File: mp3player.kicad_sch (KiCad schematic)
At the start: 7 parts, among them J1 AudioJack3, U1 ES8388, U2 ESP32-S3-WROOM-1

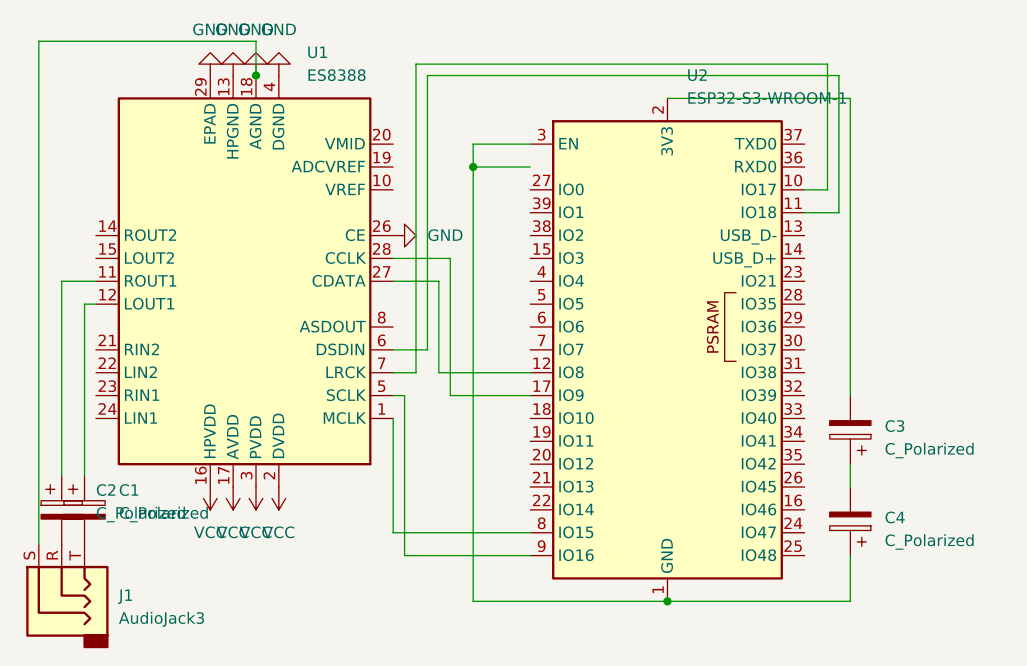
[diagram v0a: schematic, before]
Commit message: Autosave
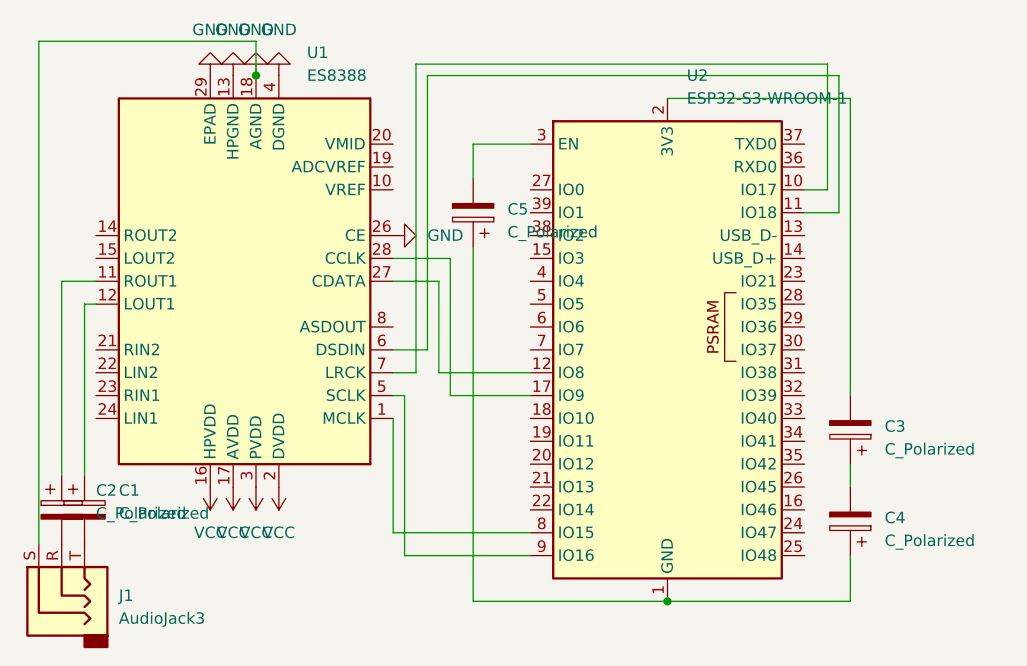
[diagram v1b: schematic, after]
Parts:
- added C5: C_Polarized, symbol Device:C_Polarized
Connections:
- net at C4.1, U2.1 (GND), U2.40 (GND)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: now also C5.1; no longer U2.3 (EN)
- new net: C5.2, U2.3 (EN)
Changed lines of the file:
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@@
-	)
-	(junction
-		(at 63.5 26.67)
-		(diameter 0)
-		(color 0 0 0 0)
 	)
 	(junction
@@
 	(wire
 		(pts
-			(xy 69.85 26.67) (xy 63.5 26.67)
-		)
-		(stroke
-			(width 0)
-			(type default)
-		)
-	)
-	(wire
-		(pts
 			(xy 54.61 36.83) (xy 60.96 36.83)
 		)
@@
 	(wire
 		(pts
-			(xy 63.5 24.13) (xy 63.5 26.67)
+			(xy 63.5 35.56) (xy 63.5 74.93)
 		)
 		(stroke
@@
 	(wire
 		(pts
-			(xy 63.5 26.67) (xy 63.5 74.93)
+			(xy 63.5 24.13) (xy 63.5 27.94)
 		)
 		(stroke
@@
 					(unit 1)
 				)
+			)
+		)
+	)
+	(symbol
+		(lib_id "Device:C_Polarized")
+		(at 63.5 31.75 180)
+		(unit 1)
+		(body_style 1)
+		(exclude_from_sim no)
+		(in_bom yes)
+		(on_board yes)
+		(in_pos_files yes)
+		(dnp no)
+		(fields_autoplaced yes)
+		(property "Reference" "C5"
+			(at 67.31 31.3689 0)
+			(show_name no)
+			(do_not_autoplace no)
+			(effects
+				(font
+					(size 1.27 1.27)
+				)
+				(justify right)
+			)
+		)
+		(property "Value" "C_Polarized"
+			(at 67.31 33.9089 0)
+			(show_name no)
+			(do_not_autoplace no)
+			(effects
+				(font
+					(size 1.27 1.27)
+				)
+				(justify right)
+			)
+		)
+		(property "Footprint" ""
+			(at 62.5348 27.94 0)
+			(hide yes)
+			(show_name no)
+			(do_not_autoplace no)
+			(effects
+				(font
+					(size 1.27 1.27)
+				)
+			)
+		)
+		(property "Datasheet" ""
+			(at 63.5 31.75 0)
+			(hide yes)
+			(show_name no)
+			(do_not_autoplace no)
+			(effects
+				(font
+					(size 1.27 1.27)
+				)
+			)
+		)
+		(property "Description" "Polarized capacitor"
+			(at 63.5 31.75 0)
+			(hide yes)
+			(show_name no)
+			(do_not_autoplace no)
+			(effects
+				(font
+					(size 1.27 1.27)
+				)
+			)
+		)
+		(pin "1"
+		)
+		(pin "2"
+		)
+		(instances
+			(project "mp3player"
+				(path "/7851373b-cb7e-4e42-801a-d8b5ac5735f4"
+					(reference "C5")
+					(unit 1)
+				)

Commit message: Autosave
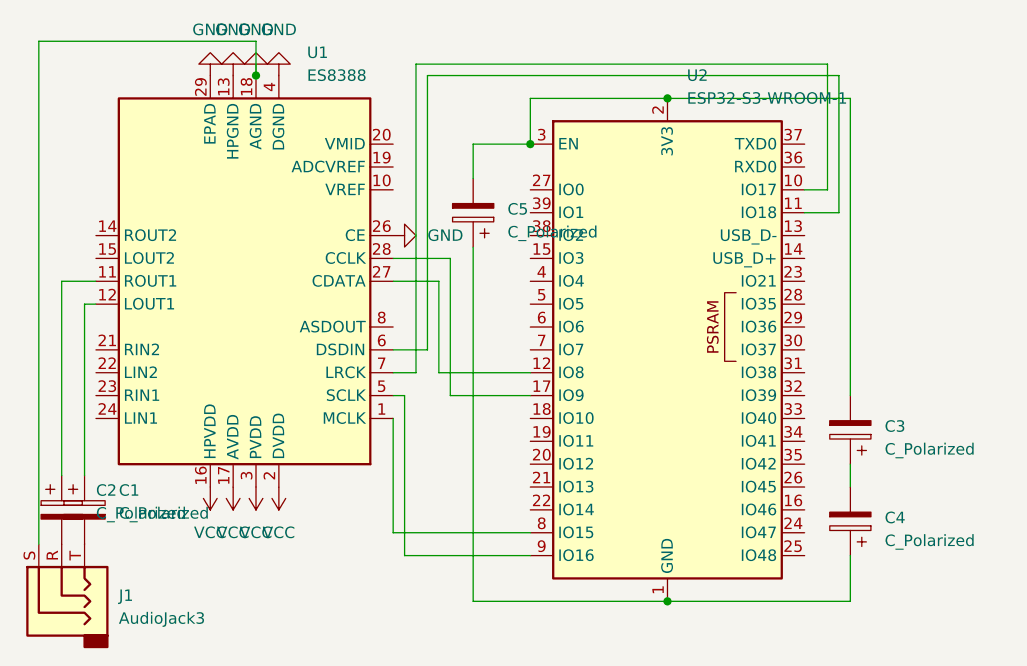
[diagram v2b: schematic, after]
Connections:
- net at C5.2, U2.3 (EN): now also C3.2, U2.2 (3V3)
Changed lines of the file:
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@@
 	(paper "A4")
 	(junction
+		(at 85.09 19.05)
+		(diameter 0)
+		(color 0 0 0 0)
+	)
+	(junction
 		(at 39.37 16.51)
 		(diameter 0)
@@
 	)
 	(junction
+		(at 69.85 24.13)
+		(diameter 0)
+		(color 0 0 0 0)
+	)
+	(junction
 		(at 85.09 74.93)
 		(diameter 0)
@@
 	(wire
 		(pts
+			(xy 69.85 19.05) (xy 85.09 19.05)
+		)
+		(stroke
+			(width 0)
+			(type default)
+		)
+	)
+	(wire
+		(pts
 			(xy 100.33 31.75) (xy 104.14 31.75)
 		)
@@
 		)
 		(stroke
+			(width 0)
+			(type default)
+		)
+	)
+	(wire
+		(pts
+			(xy 69.85 24.13) (xy 69.85 19.05)
+		)
+		(stroke

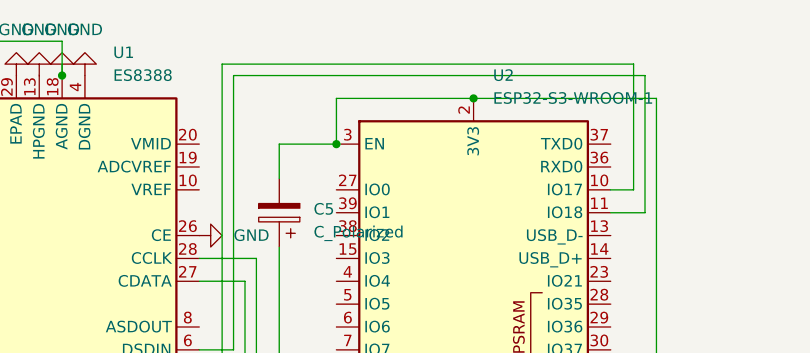
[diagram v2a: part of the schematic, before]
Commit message: Autosave
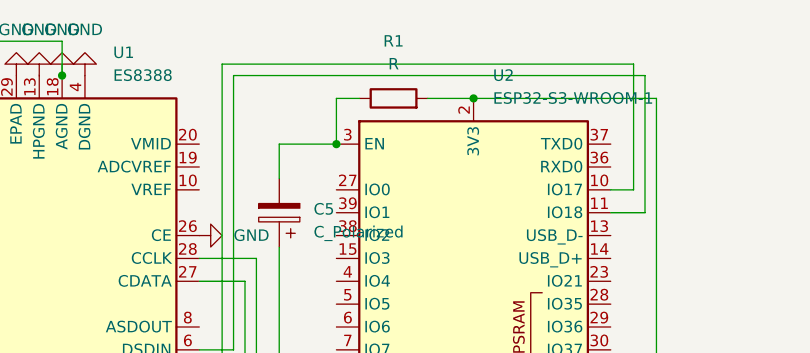
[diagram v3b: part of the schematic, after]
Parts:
- added R1: R, symbol Device:R
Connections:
- net at C5.2, U2.3 (EN): now also R1.1; no longer C3.2, U2.2 (3V3)
- new net: C3.2, R1.2, U2.2 (3V3)
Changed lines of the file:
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@@
 	(wire
 		(pts
-			(xy 69.85 19.05) (xy 85.09 19.05)
+			(xy 69.85 19.05) (xy 72.39 19.05)
 		)
 		(stroke
@@
 		(pts
 			(xy 63.5 24.13) (xy 63.5 27.94)
+		)
+		(stroke
+			(width 0)
+			(type default)
+		)
+	)
+	(wire
+		(pts
+			(xy 80.01 19.05) (xy 85.09 19.05)
 		)
 		(stroke
@@
 					(unit 1)
 				)
+			)
+		)
+	)
+	(symbol
+		(lib_id "Device:R")
+		(at 76.2 19.05 90)
+		(unit 1)
+		(body_style 1)
+		(exclude_from_sim no)
+		(in_bom yes)
+		(on_board yes)
+		(in_pos_files yes)
+		(dnp no)
+		(fields_autoplaced yes)
+		(property "Reference" "R1"
+			(at 76.2 12.7 90)
+			(show_name no)
+			(do_not_autoplace no)
+			(effects
+				(font
+					(size 1.27 1.27)
+				)
+			)
+		)
+		(property "Value" "R"
+			(at 76.2 15.24 90)
+			(show_name no)
+			(do_not_autoplace no)
+			(effects
+				(font
+					(size 1.27 1.27)
+				)
+			)
+		)
+		(property "Footprint" ""
+			(at 76.2 20.828 90)
+			(hide yes)
+			(show_name no)
+			(do_not_autoplace no)
+			(effects
+				(font
+					(size 1.27 1.27)
+				)
+			)
+		)
+		(property "Datasheet" ""
+			(at 76.2 19.05 0)
+			(hide yes)
+			(show_name no)
+			(do_not_autoplace no)
+			(effects
+				(font
+					(size 1.27 1.27)
+				)
+			)
+		)
+		(property "Description" "Resistor"
+			(at 76.2 19.05 0)
+			(hide yes)
+			(show_name no)
+			(do_not_autoplace no)
+			(effects
+				(font
+					(size 1.27 1.27)
+				)
+			)
+		)
+		(pin "1"
+		)
+		(pin "2"
+		)
+		(instances
+			(project "mp3player"
+				(path "/7851373b-cb7e-4e42-801a-d8b5ac5735f4"
+					(reference "R1")
+					(unit 1)
+				)

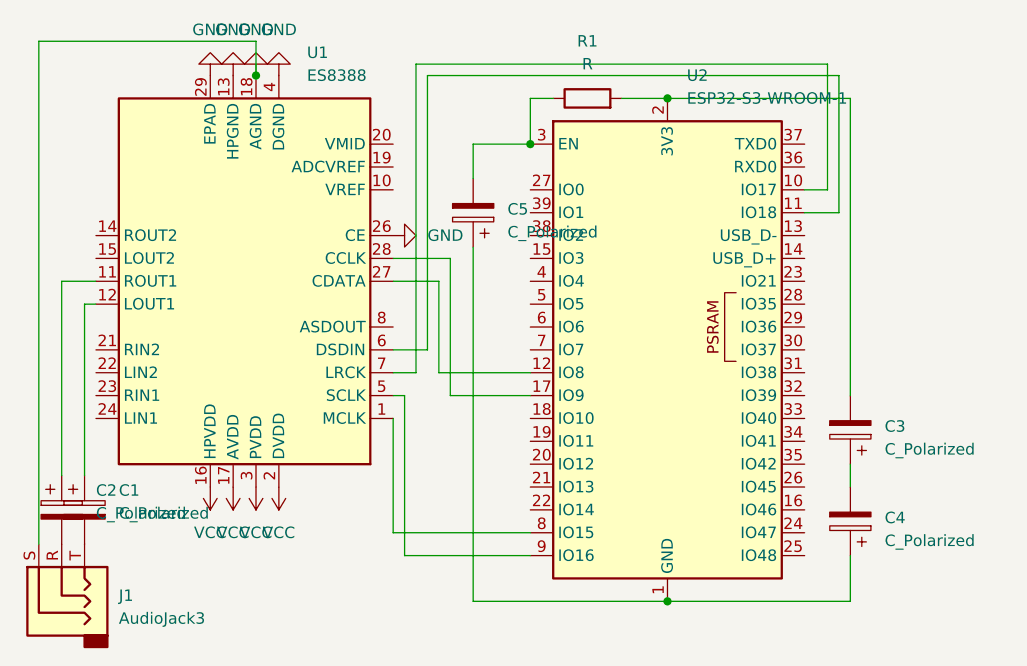
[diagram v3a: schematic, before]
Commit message: Autosave
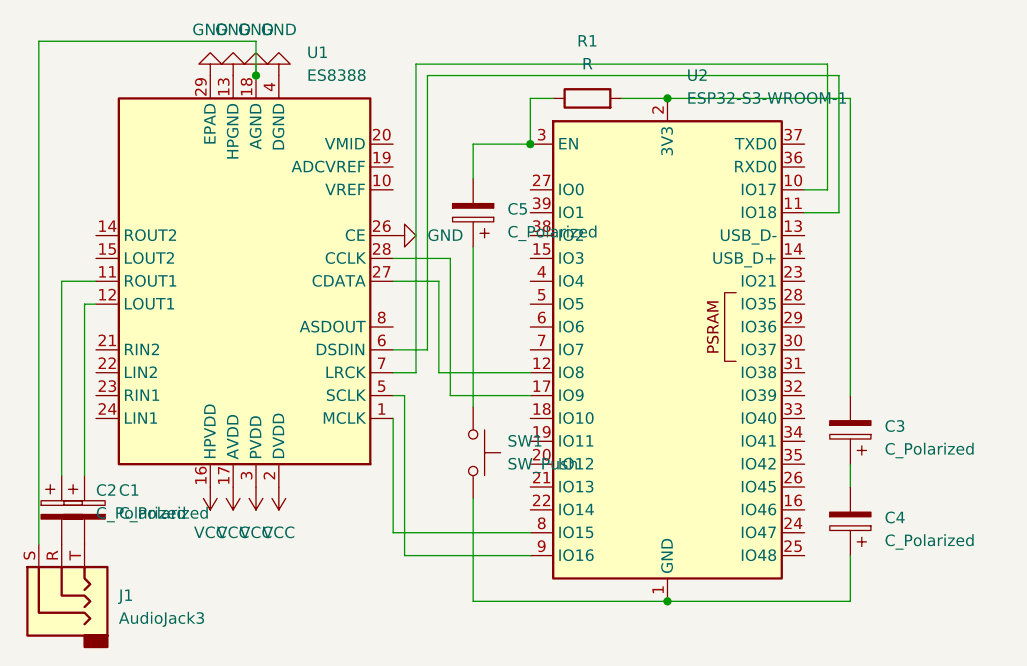
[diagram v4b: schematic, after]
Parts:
- added SW1: SW_Push, symbol Switch:SW_Push
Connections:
- net at C4.1, U2.1 (GND), U2.40 (GND)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: now also SW1.2; no longer C5.1
- new net: C5.1, SW1.1
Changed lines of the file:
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@@
+	(wire
+		(pts
+			(xy 63.5 63.5) (xy 63.5 74.93)
+		)
+		(stroke
+			(width 0)
+			(type default)
+		)
+	)
 	(wire
 		(pts
@@
 	(wire
 		(pts
-			(xy 63.5 35.56) (xy 63.5 74.93)
+			(xy 63.5 35.56) (xy 63.5 53.34)
 		)
 		(stroke
@@
 					(unit 1)
 				)
+			)
+		)
+	)
+	(symbol
+		(lib_id "Switch:SW_Push")
+		(at 63.5 58.42 270)
+		(unit 1)
+		(body_style 1)
+		(exclude_from_sim no)
+		(in_bom yes)
+		(on_board yes)
+		(in_pos_files yes)
+		(dnp no)
+		(fields_autoplaced yes)
+		(property "Reference" "SW1"
+			(at 67.31 57.1499 90)
+			(show_name no)
+			(do_not_autoplace no)
+			(effects
+				(font
+					(size 1.27 1.27)
+				)
+				(justify left)
+			)
+		)
+		(property "Value" "SW_Push"
+			(at 67.31 59.6899 90)
+			(show_name no)
+			(do_not_autoplace no)
+			(effects
+				(font
+					(size 1.27 1.27)
+				)
+				(justify left)
+			)
+		)
+		(property "Footprint" ""
+			(at 68.58 58.42 0)
+			(hide yes)
+			(show_name no)
+			(do_not_autoplace no)
+			(effects
+				(font
+					(size 1.27 1.27)
+				)
+			)
+		)
+		(property "Datasheet" ""
+			(at 68.58 58.42 0)
+			(hide yes)
+			(show_name no)
+			(do_not_autoplace no)
+			(effects
+				(font
+					(size 1.27 1.27)
+				)
+			)
+		)
+		(property "Description" "Push button switch, generic, two pins"
+			(at 63.5 58.42 0)
+			(hide yes)
+			(show_name no)
+			(do_not_autoplace no)
+			(effects
+				(font
+					(size 1.27 1.27)
+				)
+			)
+		)
+		(pin "1"
+		)
+		(pin "2"
+		)
+		(instances
+			(project "mp3player"
+				(path "/7851373b-cb7e-4e42-801a-d8b5ac5735f4"
+					(reference "SW1")
+					(unit 1)
+				)
